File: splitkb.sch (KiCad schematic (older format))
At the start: 67 parts, among them J1 MJ-4PP-9, K1 KEYSW, SW1 SW_PUSH, SW10 SW_PUSH, SW11 SW_PUSH, SW12 SW_PUSH, SW13 SW_PUSH, SW14 SW_PUSH, SW15 SW_PUSH, SW16 SW_PUSH, SW17 SW_PUSH, SW18 SW_PUSH, SW19 SW_PUSH, SW2 SW_PUSH, SW20 SW_PUSH, SW21 SW_PUSH, SW22 SW_PUSH, SW23 SW_PUSH, SW24 SW_PUSH, SW25 SW_PUSH, SW26 SW_PUSH, SW27 SW_PUSH, SW28 SW_PUSH, SW29 SW_PUSH, SW3 SW_PUSH, SW30 SW_PUSH, SW31 SW_PUSH, SW32 SW_PUSH, SW4 SW_PUSH, SW5 SW_PUSH, SW6 SW_PUSH, SW7 SW_PUSH, SW8 SW_PUSH, SW9 SW_PUSH, U1 ProMicro

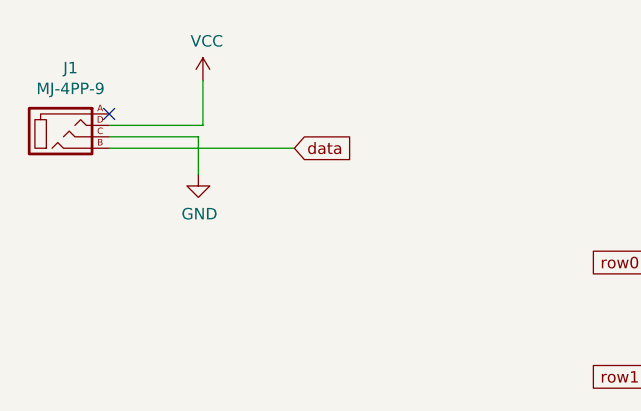
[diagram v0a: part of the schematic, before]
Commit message: minor adjustments
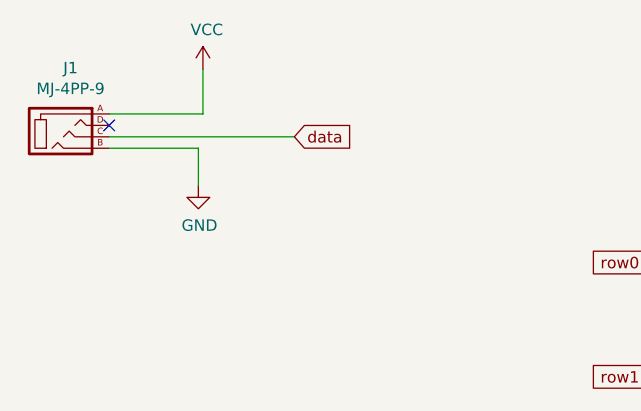
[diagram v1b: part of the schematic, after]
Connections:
- net GND: now also J1.B; no longer J1.C
- net VCC: now also J1.A; no longer J1.D
- net data: now also J1.C; no longer J1.B
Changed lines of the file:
@@
 L power:VCC #PWR0105
 U 1 1 5EFE2D39
-P 1685 905
-F 0 "#PWR0105" H 1685 755 50  0001 C CNN
-F 1 "VCC" H 1702 1078 50  0000 C CNN
-F 2 "" H 1685 905 50  0001 C CNN
-F 3 "" H 1685 905 50  0001 C CNN
-	1    1685 905
+P 1685 855
+F 0 "#PWR0105" H 1685 705 50  0001 C CNN
+F 1 "VCC" H 1702 1028 50  0000 C CNN
+F 2 "" H 1685 855 50  0001 C CNN
+F 3 "" H 1685 855 50  0001 C CNN
+	1    1685 855
 	1    0    0    -1
 $EndComp
@@
 L power:GND #PWR0103
 U 1 1 5EFDC487
-P 1665 1315
-F 0 "#PWR0103" H 1665 1065 50  0001 C CNN
-F 1 "GND" H 1670 1142 50  0000 C CNN
-F 2 "" H 1665 1315 50  0001 C CNN
-F 3 "" H 1665 1315 50  0001 C CNN
-	1    1665 1315
-	1    0    0    -1
-$EndComp
-Wire Wire Line
-	1275 1200 2085 1200
-Text GLabel 2085 1200 2    50   Input ~ 0
+P 1665 1365
+F 0 "#PWR0103" H 1665 1115 50  0001 C CNN
+F 1 "GND" H 1670 1192 50  0000 C CNN
+F 2 "" H 1665 1365 50  0001 C CNN
+F 3 "" H 1665 1365 50  0001 C CNN
+	1    1665 1365
+	1    0    0    -1
+$EndComp
+Wire Wire Line
+	1275 1200 1665 1200
+Text GLabel 2085 1150 2    50   Input ~ 0
 data
 $Comp
@@
 	1    0    0    -1
 $EndComp
-NoConn ~ 1275 1050
-Wire Wire Line
-	1275 1100 1685 1100
-Wire Wire Line
-	1685 1100 1685 905
-Wire Wire Line
-	1275 1150 1665 1150
-Wire Wire Line
-	1665 1150 1665 1315
+NoConn ~ 1275 1100
+Wire Wire Line
+	1275 1050 1685 1050
+Wire Wire Line
+	1685 1050 1685 855
 Connection ~ 10600 3200
 Wire Wire Line
@@
 	1    0    0    -1
 $EndComp
+Wire Wire Line
+	1665 1200 1665 1365
+Wire Wire Line
+	1275 1150 2085 1150
 $EndSCHEMATC

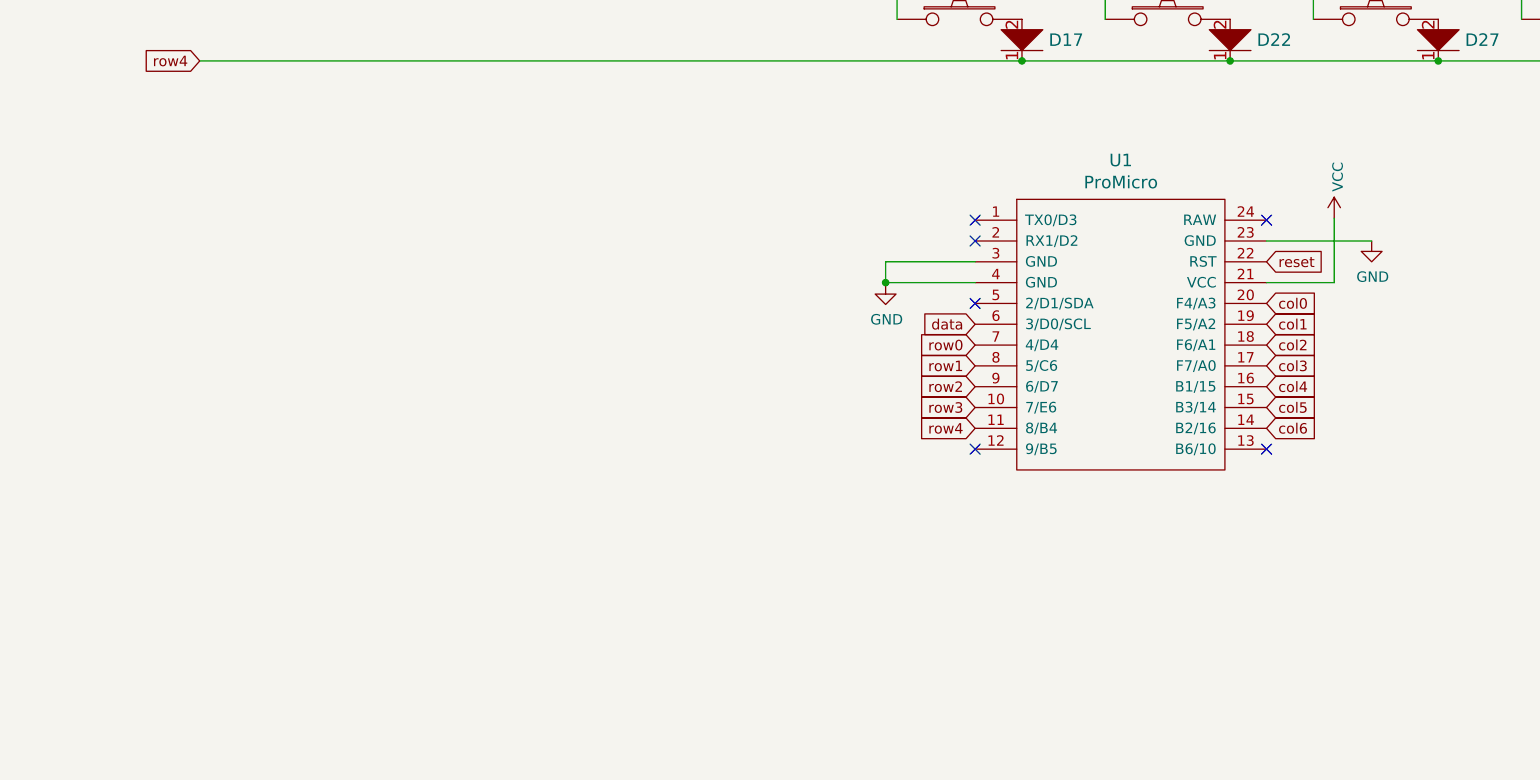
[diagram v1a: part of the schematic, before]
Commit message: test
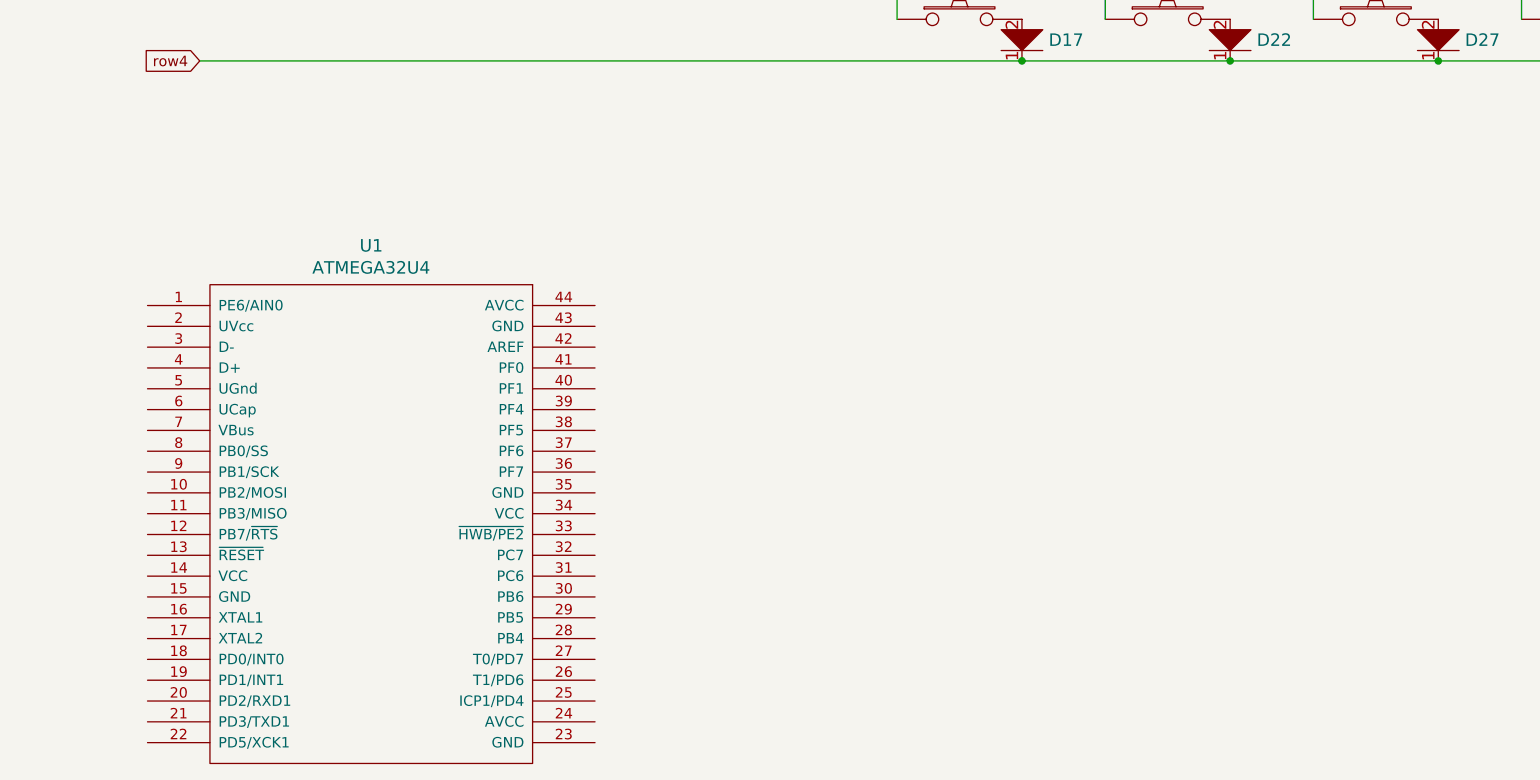
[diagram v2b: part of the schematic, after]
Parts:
- removed U1: ProMicro, kbd:ProMicro_v2, symbol kbd:ProMicro
- added U1: ATMEGA32U4, Package_QFP:LQFP-44_10x10mm_P0.8mm, symbol keyboard_parts:ATMEGA32U4
- D1, D10, D11, D12, D13, D14, D15, D16, D17, D18, D19, D2, D20, D21, D22, D23, D24, D25, D26, D27, D28, D29, D3, D30, D31, D32, D4, D5, D6, D7, D8, D9: footprint kbd:D3_TH_SMD -> Diode_SMD:D_SOD-323_HandSoldering
- J1: footprint kbd:MJ-4PP-9 -> (none)
- K1: footprint kbd:ResetSW -> random-keyboard-parts:SKQG-1155865
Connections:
- no-connect marks 7 -> 1
